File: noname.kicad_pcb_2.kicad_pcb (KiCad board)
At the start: 2 copper layers, 122.2 x 127.3 mm, 105 parts, among them P1 USB_A, SW0:1 SPACE, SW0:2 ENTER, SW0:3 ALTGR, SW0:4 FN_R, SW0:5 MOD4, SW0:6 CTRL_R, SW1:1 B, SW1:2 M, SW1:3 ,, SW1:4 ., SW1:5 J, SW1:6 END, SW2:1 S, SW2:2 N, SW2:3 R, SW2:4 T, SW2:5 D, SW2:6 Y, SW3:1 K, SW3:2 H, SW3:3 G, SW3:4 F, SW3:5 Q, SW3:6 ẞ, SW4:1 6, SW4:2 7, SW4:3 8, SW4:4 9, SW4:5 0, SW4:6 BCKSPC, U1 ATmega32U4-AU, X1 CRYSTAL

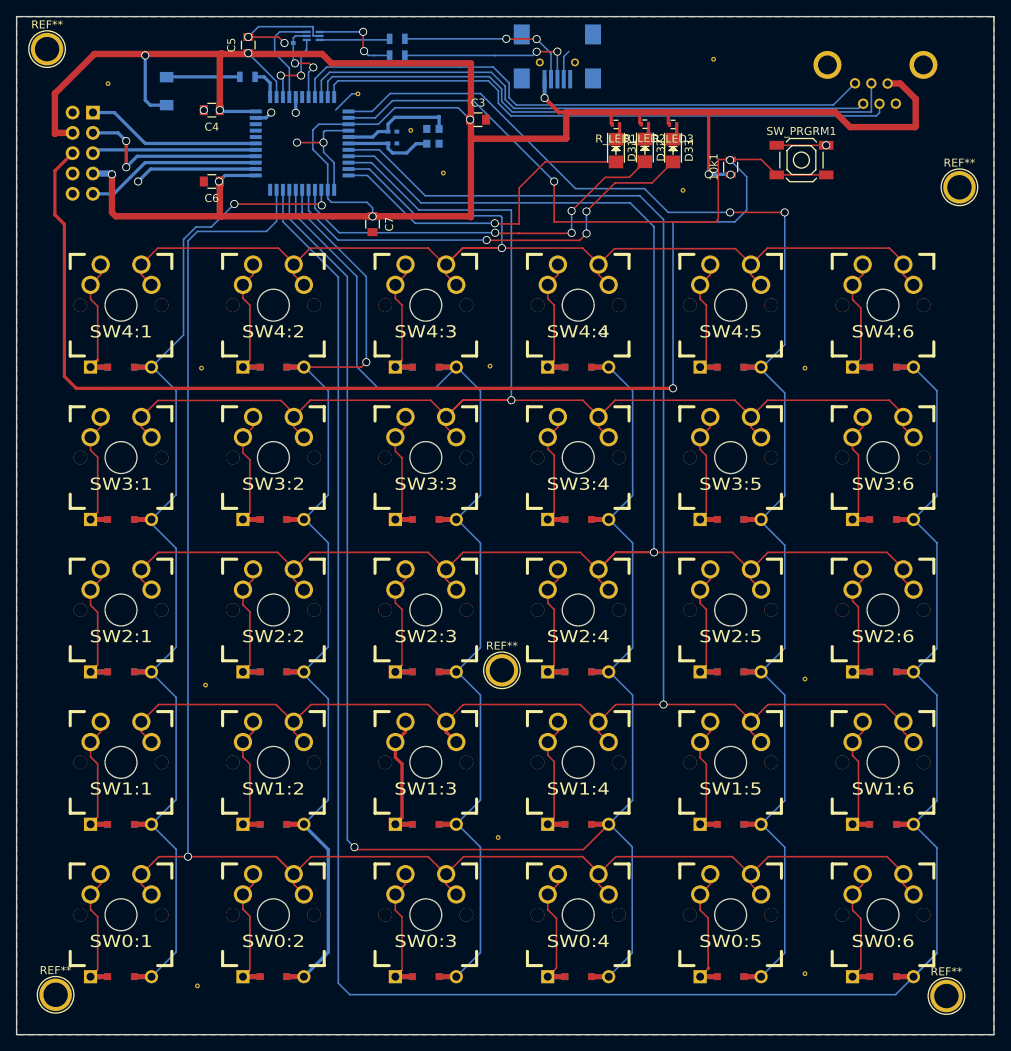
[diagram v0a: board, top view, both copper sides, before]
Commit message: some footprints and track redraw
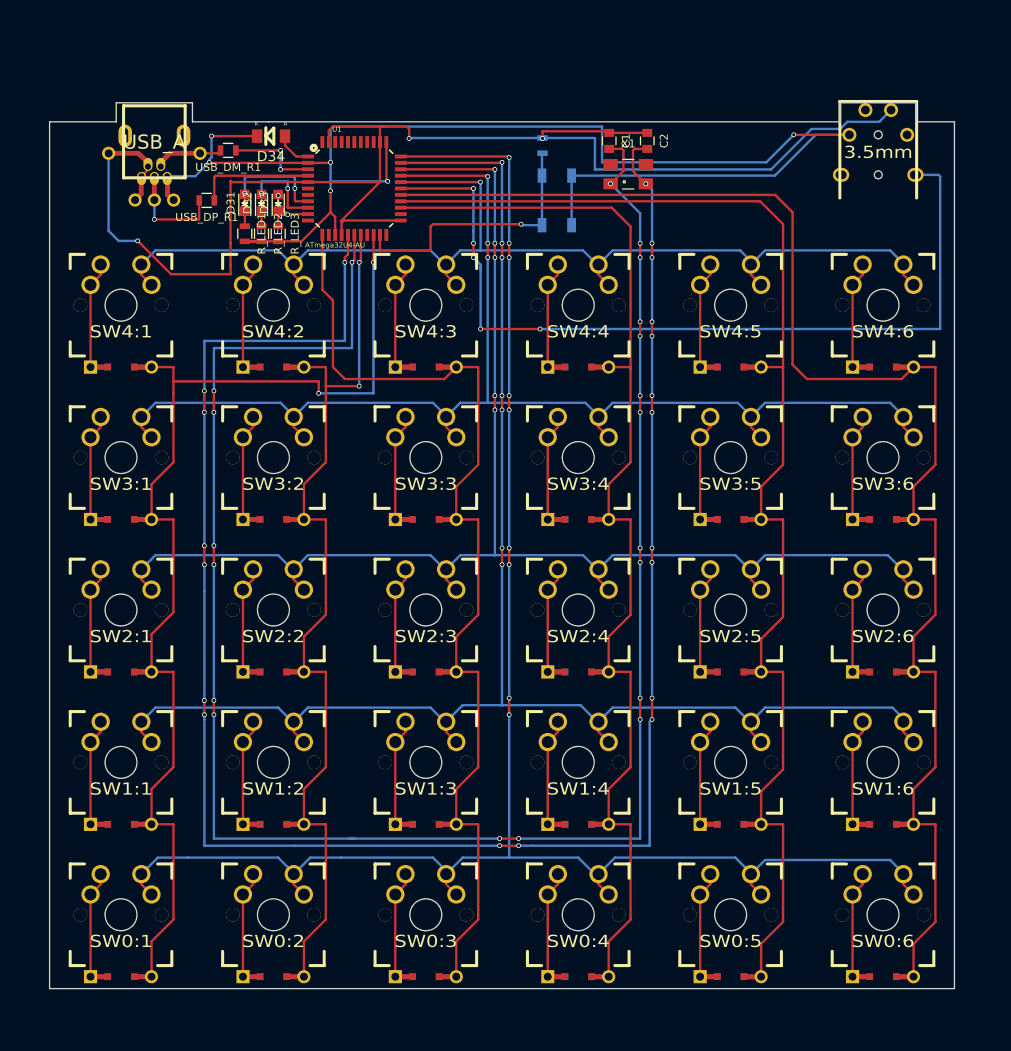
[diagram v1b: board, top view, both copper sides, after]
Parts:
- removed 100nF1: CBUS, Capacitors_SMD:C_0402
- removed C3, C4, C5, C6, C7: C, Capacitors_SMD:C_0805
- removed DZ1: USBLC6-2P6, mmmm:usblc6-2p6
- removed JTAG1: JTAG, aud:IDC_Header_Straight_10pins
- removed REF** (x14): VIA6MM, mmmm:VIA6MM
- removed REF** (x5): 1pin, Connect:1pin
- removed RJ11: CONN_6, mmmm:rj11
- removed VCCCHECK1: R47k, Resistors_SMD:R_0805
- added K1: XLR3, footprint:4pin35mmAudio, B.Cu at (126.5, 35.1)
- 10k1, SW_PRGRM1: moved to B.Cu
- C1, C2: footprint Capacitors_SMD:C_0402 -> Capacitors_SMD:C_0805; moved to F.Cu
- D31, D32, D33: footprint LEDs:LED_1206 -> LEDs:LED_0805
- D34: footprint Diodes_SMD:MiniMELF_Standard -> diode smd:Diode-MiniMELF_Standard_RevA_27July2010; moved to F.Cu
- P1: footprint mmmm:usb-b-mini-female -> footprint:USBMINImod; moved to F.Cu
- R_LED1, R_LED2, R_LED3: footprint Resistors_SMD:R_0402 -> Resistors_SMD:R_0805
- U1, USB_DM_R1, USB_DP_R1: moved to F.Cu
- X1: footprint Crystals:Crystal_SMD_2520_4Pads -> Crystals:Crystal_SMD_0603_4Pads; moved to F.Cu
- moved P1 52.1 mm to (36.0, 25.6)
- moved R_LED3 51.2 mm to (51.5, 39.6), turned to 270 degrees
- moved R_LED2 49.8 mm to (49.4, 39.6), turned to 270 degrees
- moved D33 49.8 mm to (51.5, 35.7), turned to 90 degrees
- moved D32 48.4 mm to (49.4, 35.7), turned to 90 degrees
- moved R_LED1 48.4 mm to (47.3, 39.6), turned to 270 degrees
- moved D31 46.8 mm to (47.3, 35.7), turned to 90 degrees
- moved C2 31.9 mm to (97.6, 28.0), turned to 270 degrees
- moved SW_PRGRM1 31.0 mm to (86.3, 35.4), turned to 270 degrees
- moved USB_DP_R1 29.9 mm to (42.6, 35.4), turned to 180 degrees
- moved C1 27.1 mm to (92.9, 28.0), turned to 270 degrees
- moved USB_DM_R1 25.3 mm to (45.2, 29.2), turned to 180 degrees
- moved X1 24.9 mm to (95.3, 32.1), turned to 0 degrees
- moved 10k1 23.7 mm to (84.5, 28.6)
- moved D34 14.2 mm to (50.6, 27.4), turned to 180 degrees
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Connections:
- 10k1 pad 1: /P14_VCC -> /PRGRM
- 10k1 pad 2: /RST -> /UGND
- D34 pad 1: Net-(D34-Pad1) -> /P1
- D34 pad 2: /P14_VCC -> /UVCC
- P1 pad 1: /P14_VCC -> /UVCC
- R_LED1 pad 2: /P14_VCC -> /UVCC
- R_LED2 pad 2: /P14_VCC -> /UVCC
- R_LED3 pad 2: /P14_VCC -> /UVCC
- SW_PRGRM1 pad 1: /UGND -> /PRGRM
- SW_PRGRM1 pad 2: /RST -> /UVCC
- U1 pad 10: /DATA1 -> /LED3
- U1 pad 11: /DATA2 -> (no net)
- U1 pad 12: /COL4 -> /COL2
- U1 pad 13: /RST -> (no net)
- U1 pad 14: /P14_VCC -> /UVCC
- U1 pad 18: /ROW1 -> /COL1
- U1 pad 19: /ROW2 -> (no net)
- U1 pad 2: /P14_VCC -> /UVCC
- U1 pad 20: /ROW3 -> /COL0
- U1 pad 21: /ROW4 -> /PRGRM
- U1 pad 22: /LED1 -> (no net)
- U1 pad 24: /P14_VCC -> (no net)
- U1 pad 25: /COL0 -> /COL3
- U1 pad 26: /LED2 -> /COL4
- U1 pad 27: /LED3 -> /COL5
- U1 pad 28: /COL1 -> /DATA
- U1 pad 29: /COL2 -> /ROW4
- U1 pad 3: /D-in -> /USB_DM
- U1 pad 30: /COL3 -> /ROW3
- U1 pad 31: /COL5 -> /ROW2
- U1 pad 32: /ROW0 -> /ROW1
- U1 pad 33: (no net) -> /ROW0
- U1 pad 34: /P14_VCC -> /UVCC
- U1 pad 36: /TDI -> (no net)
- U1 pad 37: /TDO -> (no net)
- U1 pad 38: /TMS -> (no net)
- U1 pad 39: /TCK -> (no net)
- U1 pad 4: /D+in -> /USB_DP
- U1 pad 44: /P14_VCC -> (no net)
- U1 pad 7: /VBus -> (no net)
- U1 pad 8: /SS -> /LED1
- U1 pad 9: /SCLK -> /LED2
- USB_DM_R1 pad 1: /D-out -> /USB_DM
- USB_DP_R1 pad 1: /D+out -> /USB_DP
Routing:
- net /P14_VCC: track 301.1 -> 0.00 mm, vias 10 -> 0
- net /XTAL1: track 11.1 -> 237.1 mm, vias 0 -> 20
- net /XTAL2: track 14.5 -> 239.6 mm, vias 0 -> 20
- net /RST: track 222.3 -> 0.00 mm, vias 3 -> 0
- net /UVCC: track 0.00 -> 187.6 mm, vias 0 -> 6
- net /UGND: track 63.2 -> 186.5 mm, vias 9 -> 3
- net /DATA: track 0.00 -> 107.0 mm, vias 0 -> 5
- net /COL5: track 265.6 -> 177.1 mm
- net /DATA1: track 76.5 -> 0.00 mm
- net /SS: track 74.6 -> 0.00 mm
- net /DATA2: track 73.9 -> 0.00 mm
- net /SCLK: track 73.3 -> 0.00 mm
- net /COL3: track 205.0 -> 140.4 mm, vias 1 -> 0
- net /LED3: track 55.4 -> 5.60 mm, vias 3 -> 2
- net /LED2: track 50.4 -> 10.7 mm, vias 3 -> 2
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- removed copper zone on B.Cu, net /UGND
- removed copper zone on F.Cu, net /UGND
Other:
- board size 122.2 x 127.3 mm -> 113.1 x 110.7 mm
- net class Default: clearance 0.152 -> 0.2; trace_width 0.4064 -> 0.3; via_dia 1.016 -> 0.6; via_drill 0.7874 -> 0.4
- net class phat added: clearance 0.2, trace_width 2, via_dia 0.6, via_drill 0.4
- rule trace_clearance: 0.152 -> 0.2
- rule trace_min: 0.152 -> 0.2
